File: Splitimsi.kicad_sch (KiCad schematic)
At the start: 44 parts, among them SW1 MX_RGB, SW10 MX_RGB, SW11 MX_RGB, SW12 RotaryEncoder_Switch, SW13 MX_RGB, SW14 MX_RGB, SW15 MX_RGB, SW16 MX_RGB, SW17 MX_RGB, SW18 MX_RGB, SW19 MX_RGB, SW2 MX_RGB, SW20 MX_RGB, SW21 MX_RGB, SW22 MX_RGB, SW23 MX_RGB, SW24 MX_RGB, SW25 MX_RGB, SW26 MX_RGB, SW27 MX_RGB, SW28 MX_RGB, SW29 MX_RGB, SW3 MX_RGB, SW30 MX_RGB, SW4 MX_RGB, SW5 MX_RGB, SW6 RotaryEncoder_Switch, SW7 MX_RGB, SW8 MX_RGB, SW9 MX_RGB, U1 ProMicro, U2 TRRS

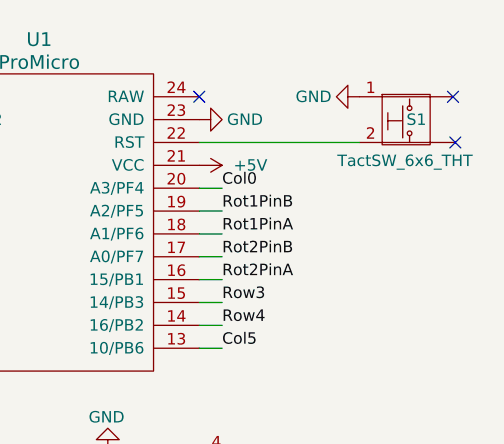
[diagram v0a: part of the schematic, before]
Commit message: reset button 3d view test
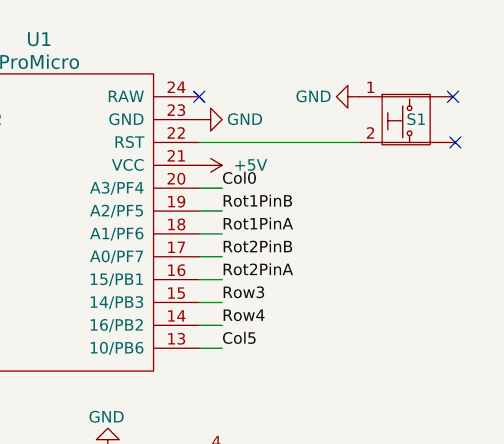
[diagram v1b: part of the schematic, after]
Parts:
- S1: value TactSW_6x6_THT -> (none); footprint aio3-misc:PushButton_6x6mm_TH_Pretty -> (none)
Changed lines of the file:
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@@
     (in_bom yes) (on_board yes)
     (property "Reference" "S1" (id 0) (at 213.36 24.13 0))
-    (property "Value" "TactSW_6x6_THT" (id 1) (at 212.09 28.702 0))
-    (property "Footprint" "aio3-misc:PushButton_6x6mm_TH_Pretty" (id 2) (at 212.09 20.066 0)
+    (property "Value" "" (id 1) (at 212.09 28.702 0))
+    (property "Footprint" "" (id 2) (at 212.09 20.066 0)
       (effects (font (size 1.27 1.27)) hide)
     )
@@
     )
     (path "/a2474201-d835-4ea6-9d62-0592a109ce48"
-      (reference "S1") (unit 1) (value "TactSW_6x6_THT") (footprint "aio3-misc:PushButton_6x6mm_TH_Pretty")
+      (reference "S1") (unit 1) (value "TactSW_6x6_THT") (footprint "Button_Switch_SMD:SW_SPST_B3U-1000P")
     )
     (path "/200aa83c-0260-4790-a345-ddeba1e13353"

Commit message: Update Splitimsi.kicad_sch
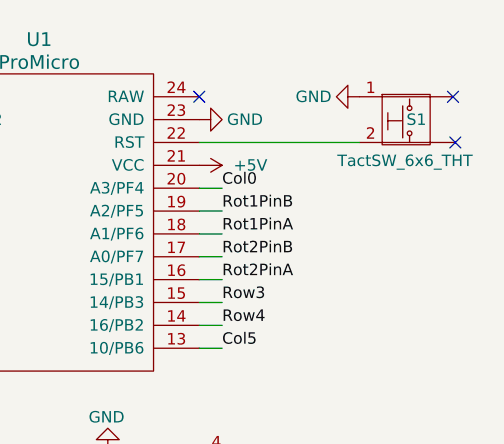
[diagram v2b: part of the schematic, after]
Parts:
- S1: value (none) -> TactSW_6x6_THT; footprint (none) -> Button_Switch_SMD:SW_SPST_B3U-1000P
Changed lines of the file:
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@@
     (in_bom yes) (on_board yes)
     (property "Reference" "S1" (id 0) (at 213.36 24.13 0))
-    (property "Value" "" (id 1) (at 212.09 28.702 0))
-    (property "Footprint" "" (id 2) (at 212.09 20.066 0)
+    (property "Value" "TactSW_6x6_THT" (id 1) (at 212.09 28.702 0))
+    (property "Footprint" "Button_Switch_SMD:SW_SPST_B3U-1000P" (id 2) (at 212.09 20.066 0)
       (effects (font (size 1.27 1.27)) hide)
     )
